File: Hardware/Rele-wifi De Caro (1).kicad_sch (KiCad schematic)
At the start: 38 parts, among them IC1 MC7805CD2TG, J1 Screw_Terminal_01x03, J2 Screw_Terminal_01x03, J3 Screw_Terminal_01x03, J4 Screw_Terminal_01x03, J5 Screw_Terminal_01x02, K1 PR13-5V-450-1C, K2 PR13-5V-450-1C, K3 PR13-5V-450-1C, K4 PR13-5V-450-1C, Q1 PC817-B, Q2 PC817-B, Q3 BC547, Q4 BC547, Q5 PC817-B, Q6 BC547, Q7 PC817-B, Q8 BC547, SW1 SW_DPST_x2, U2 ESP32-CAM

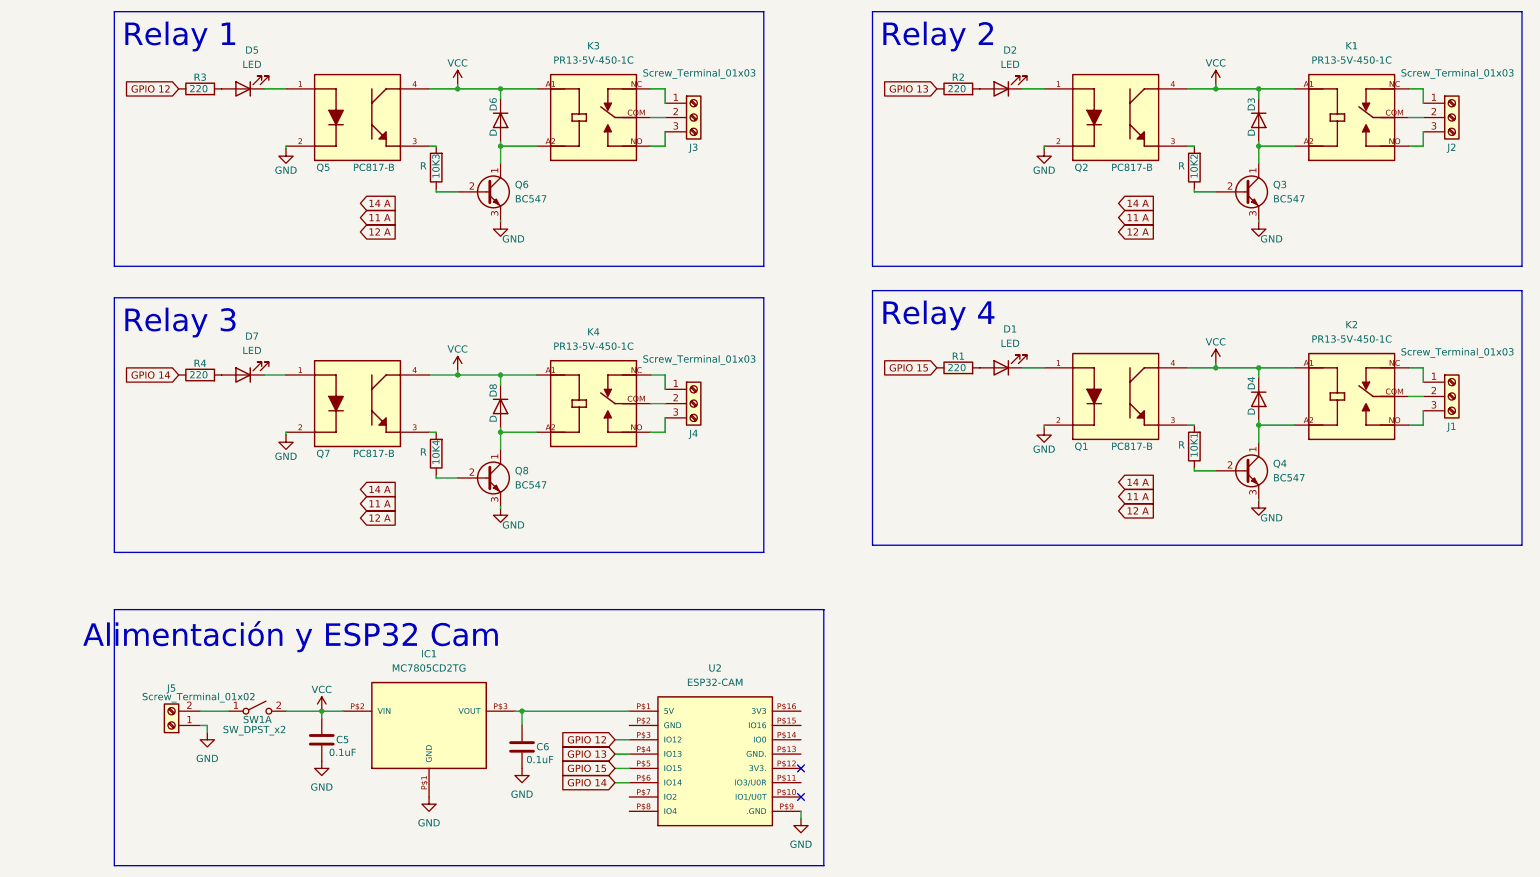
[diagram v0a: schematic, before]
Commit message: PCB casi terminado
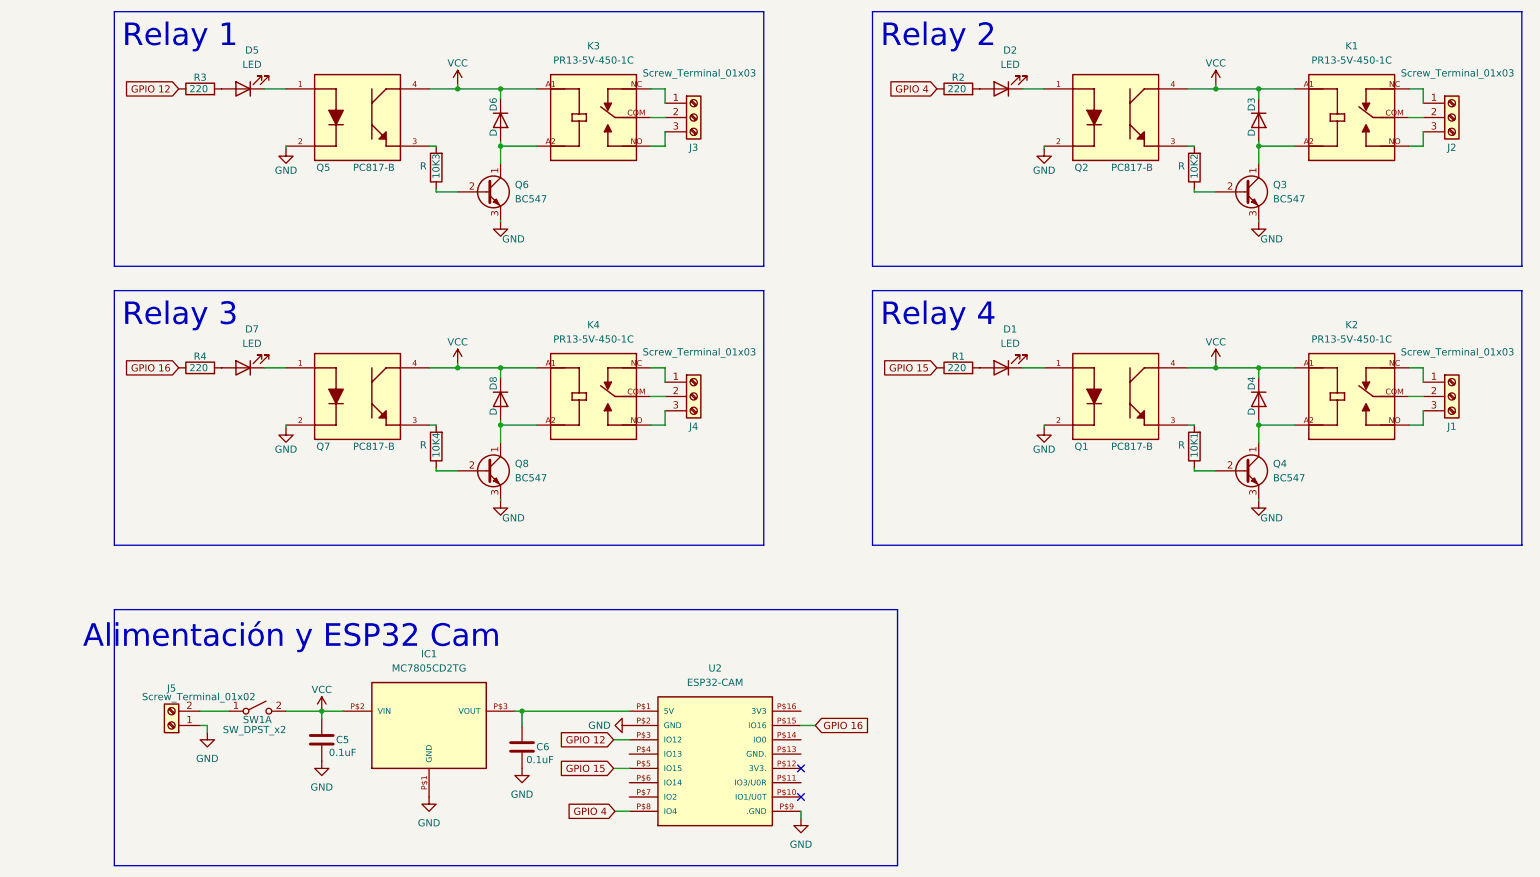
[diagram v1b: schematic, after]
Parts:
- D3, D4, D6, D8: footprint Diode_SMD:D_0805_2012Metric -> Diode_SMD:D_SMA
- SW1: footprint (none) -> Connector_PinHeader_2.54mm:PinHeader_1x02_P2.54mm_Vertical
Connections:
- net GND: now also U2.P$2 (GND)
- net GPIO 16: now reaches U2.P$15 (IO16)
- net GPIO 16: now also R4.1
- net GPIO 4: now reaches U2.P$8 (IO4)
- net GPIO 4: now also R2.1
- net GPIO 13: no longer names the net of U2.P$4 (IO13)
- net GPIO 13: no longer R2.1
- net GPIO 14: no longer names the net of U2.P$6 (IO14)
- net GPIO 14: no longer R4.1
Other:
- moved on the sheet: 10K4, D7, D8, J4, K4, Q7, Q8, R4
